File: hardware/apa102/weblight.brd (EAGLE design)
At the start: 31.8 x 12 mm, 16 parts, among them U1 ATtiny85-20SU

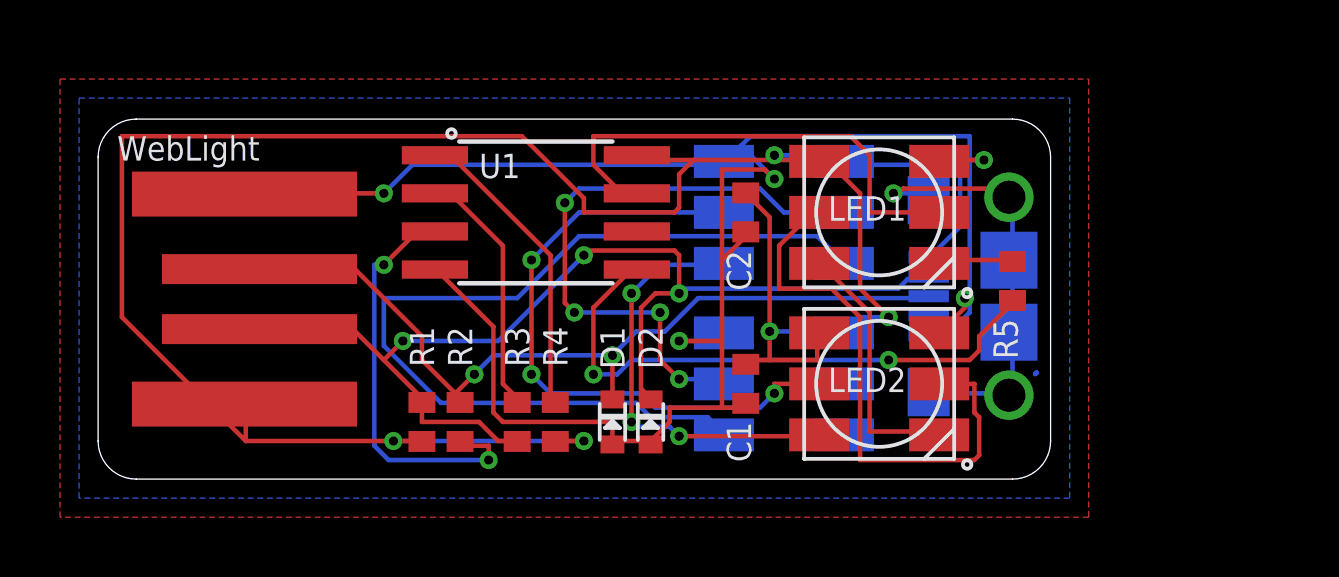
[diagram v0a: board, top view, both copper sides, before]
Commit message: a-mf1
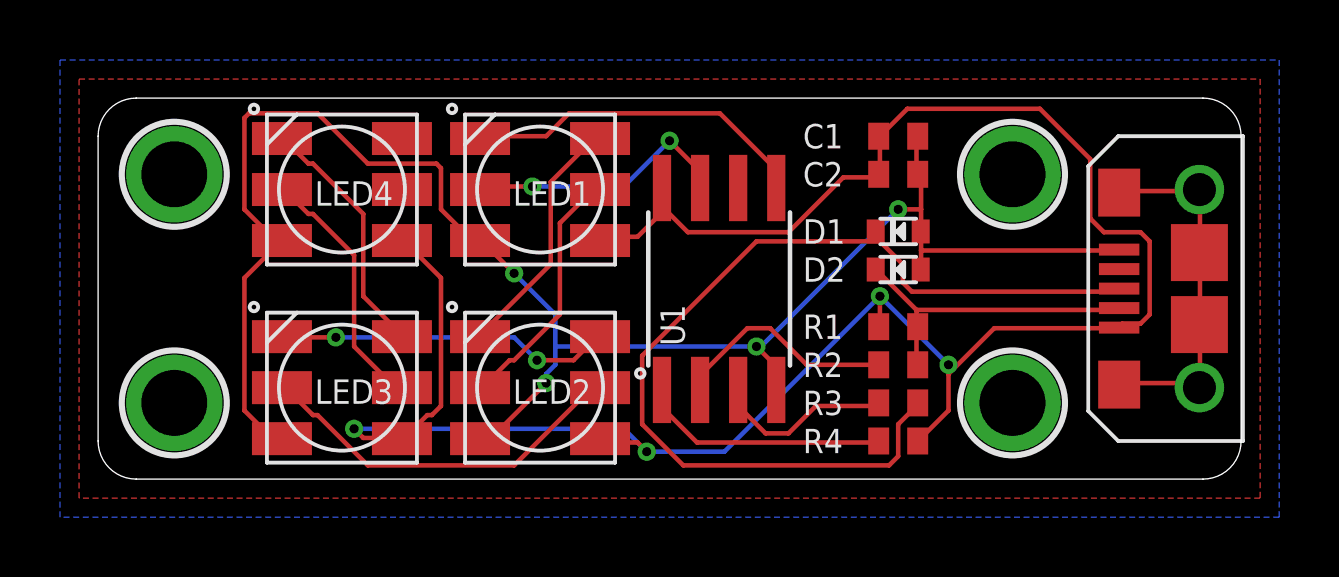
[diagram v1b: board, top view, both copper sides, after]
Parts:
- removed JP-USB-TOP: USBPCB, SparkFun-Connectors:USB-A-PCB
- removed R5: 470, rcl:R0402
- added HOLE1, HOLE2, HOLE3, HOLE4: MOUNTINGHOLE2.0, microbuilder:MOUNTINGHOLE_2.0_PLATED
- C1: value 10uF -> 1uF
- moved R1 16.2 mm to (26.7, 5.08), turned to 0 degrees
- moved LED4 16.1 mm to (8.13, 9.65), flipped to the top, turned to 180 degrees
- moved LED3 15.8 mm to (8.13, 3.05), flipped to the top, turned to 180 degrees
- moved R2 14.7 mm to (26.7, 3.81), turned to 180 degrees
- moved R3 12.7 mm to (26.7, 2.54), turned to 0 degrees
- moved D1 11.4 mm to (26.7, 8.26), turned to 90 degrees
- moved R4 11.4 mm to (26.7, 1.27), turned to 180 degrees
- moved LED1 11.3 mm to (14.7, 9.65), turned to 180 degrees
- moved LED2 11.3 mm to (14.7, 3.05), turned to 180 degrees
- moved D2 9.69 mm to (26.7, 6.99), turned to 90 degrees
- moved C1 9.69 mm to (26.7, 11.4), turned to 180 degrees
- moved U1 6.60 mm to (20.7, 6.35), turned to 0 degrees
- moved JP-USB-MICRO 6.36 mm to (35.3, 6.35), flipped to the top, turned to 90 degrees
- moved C2 5.24 mm to (26.7, 10.2), turned to 180 degrees
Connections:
- removed net DIN_RAW: R5.2, U1.5
- net DIN_1: now also U1.5; no longer R5.1
- net GND: now also C1.1, C2.1; no longer C1.2, C2.2, JP-USB-TOP.GND
- net USB_D_MINUS: now also R2.2; no longer R3.2
- net USB_D_MINUS_RAW: now also R1.2, R2.1; no longer JP-USB-TOP.USB_M, R1.1, R3.1
- net USB_D_PLUS: now also R3.1; no longer R2.2
- net USB_D_PLUS_RAW: now also R3.2; no longer JP-USB-TOP.USB_P, R2.1
- net VCC: now also C1.2, C2.2, R1.1; no longer C1.1, C2.1, JP-USB-TOP.5V, R1.2
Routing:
- net USB_D_MINUS_RAW: track 36.6 -> 10.6 mm, vias 3 -> 0
- net DIN_4: track 30.7 -> 8.36 mm
- net DIN_RAW: track 19.5 -> 0.00 mm, vias 2 -> 0
- net CLK_4: track 20.5 -> 8.51 mm, vias 4 -> 0
- net CLK_2: track 18.7 -> 8.60 mm
- net GND: track 68.8 -> 59.0 mm, vias 5 -> 4
- net VCC: track 84.2 -> 74.5 mm, vias 5 -> 4
- net DIN_1: track 2.56 -> 11.6 mm
- net CLK_3: track 21.4 -> 12.8 mm, vias 3 -> 0
- net USB_D_PLUS: track 14.1 -> 6.01 mm, vias 2 -> 0
- net CLK_1: track 16.5 -> 9.02 mm, vias 0 -> 2
- net USB_D_PLUS_RAW: track 28.0 -> 33.0 mm, vias 2 -> 0
- net SLD: track 15.2 -> 12.1 mm, vias 1 -> 0
- net DIN_3: track 14.2 -> 11.2 mm, vias 3 -> 2
- net N_RESET: track 10.2 -> 8.31 mm
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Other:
- board size 31.8 x 12 mm -> 38.1 x 12.7 mm
- board text removed: "sowbug.github.io/weblight"
